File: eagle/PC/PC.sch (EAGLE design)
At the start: 13 parts

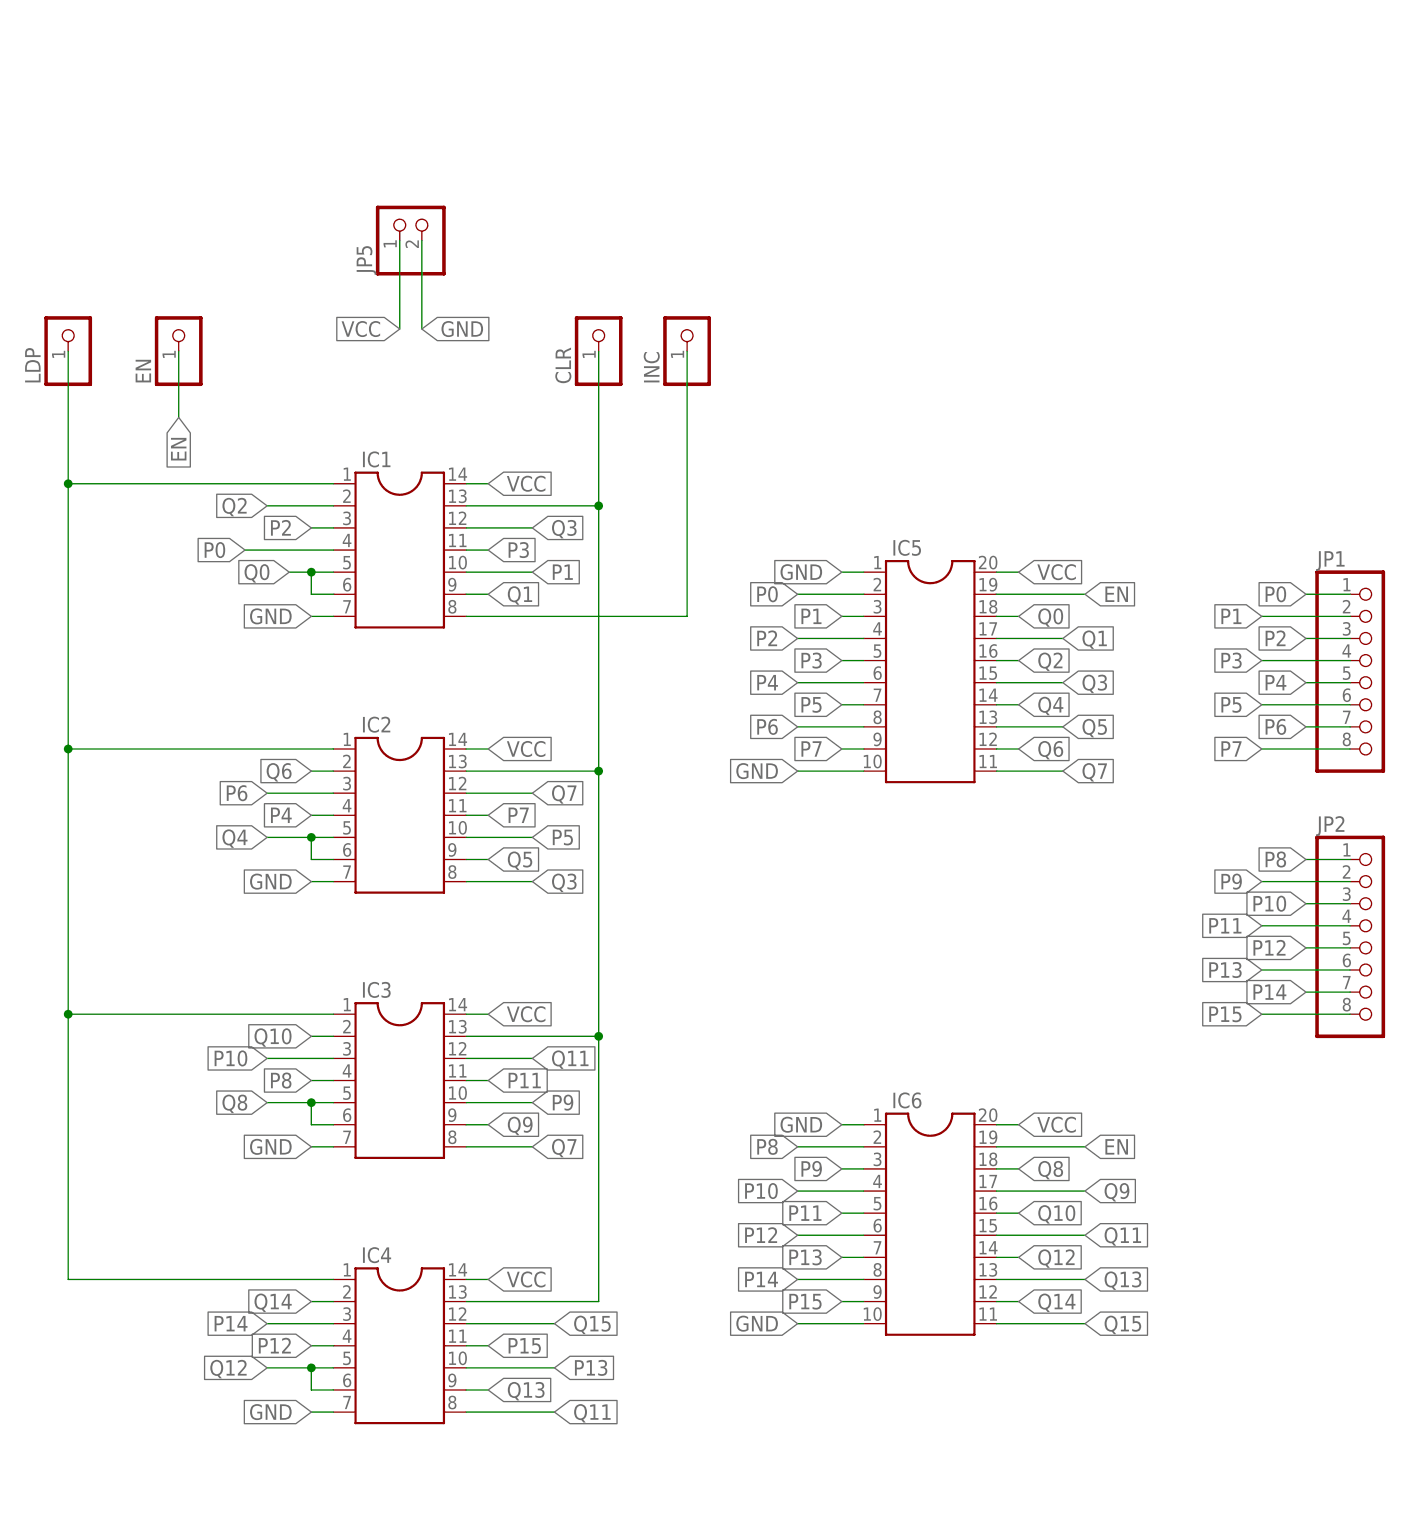
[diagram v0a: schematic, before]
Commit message: Redo PC.
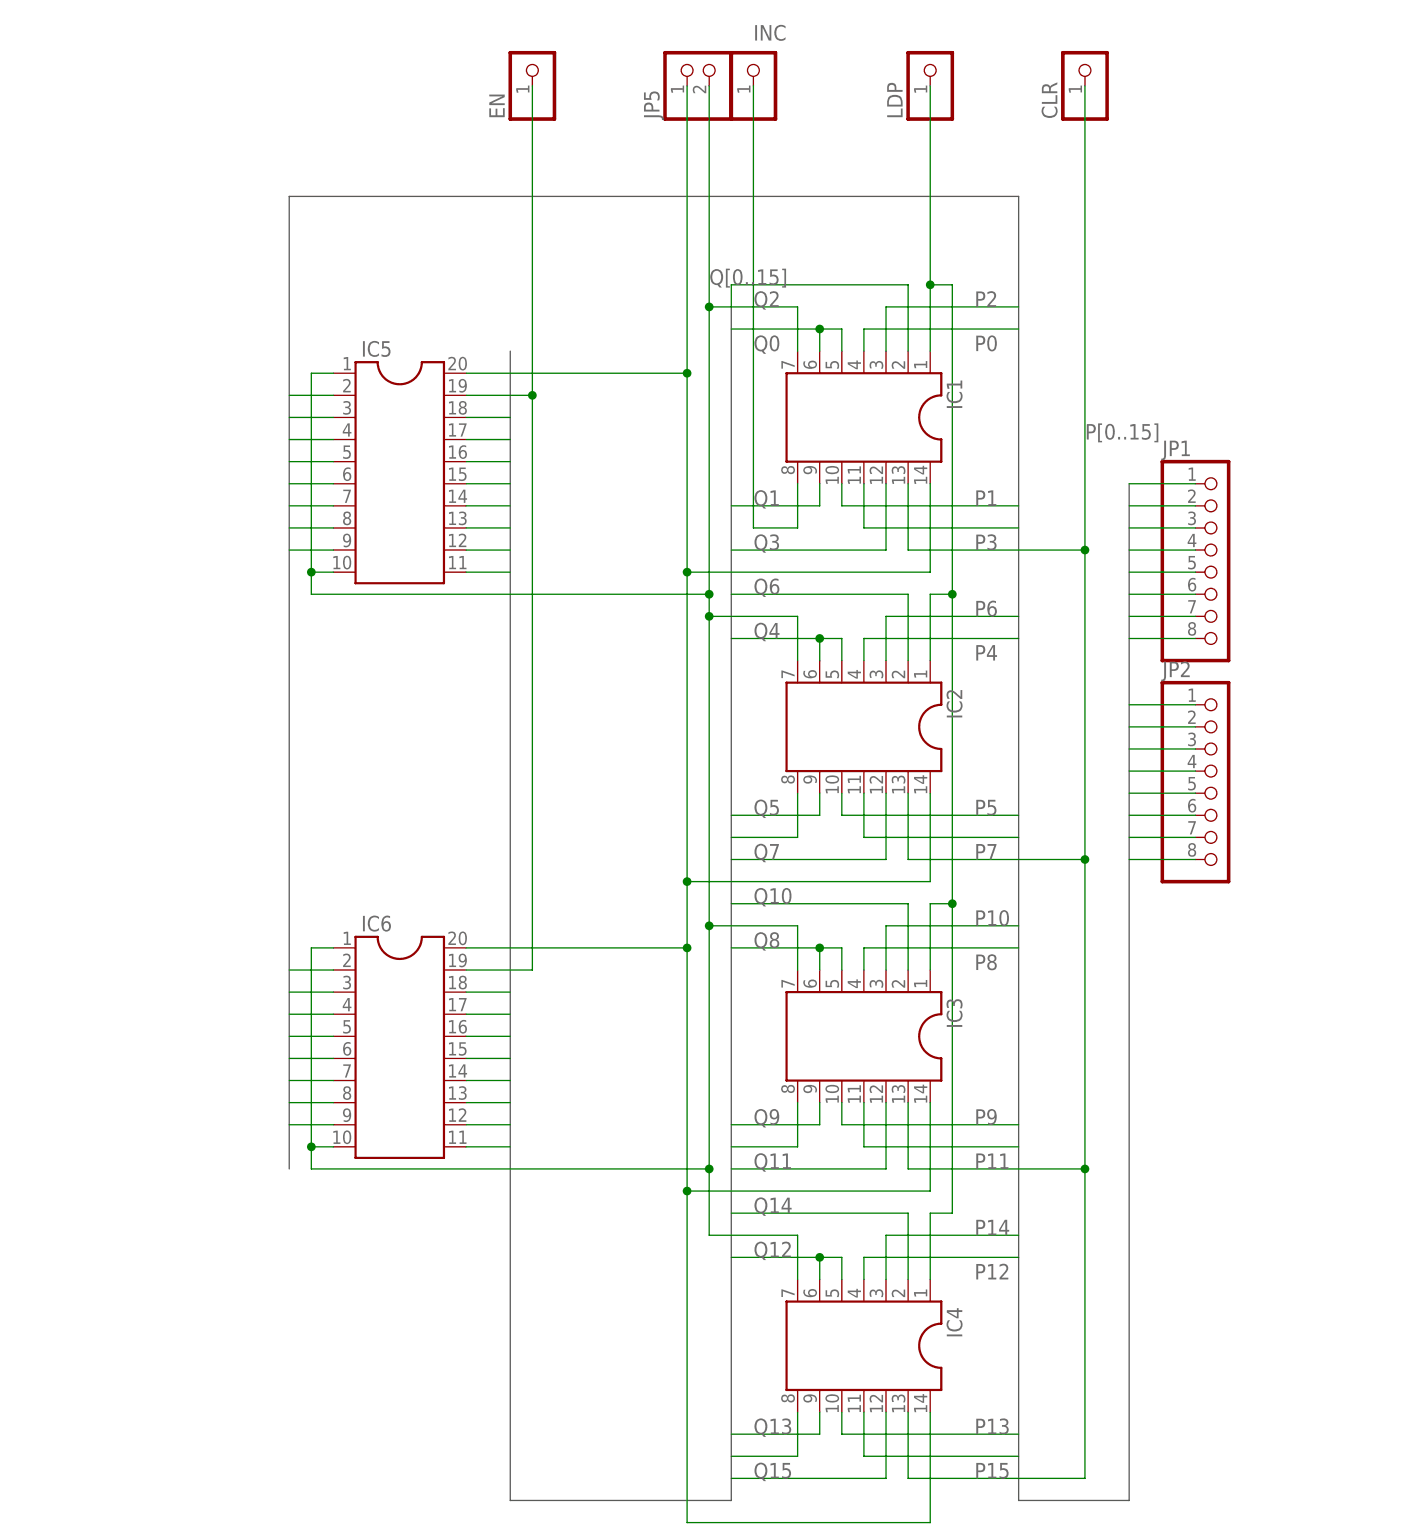
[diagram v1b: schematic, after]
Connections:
- net EN renamed N$5
- net GND renamed N$3
- net VCC renamed N$7
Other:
- moved on the sheet: CLR, EN, IC1, IC2, IC3, IC4, IC5, IC6, INC, JP1, JP2, JP5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
